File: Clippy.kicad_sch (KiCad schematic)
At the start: 17 parts, among them J1 Conn_01x08, SW1 PEC11R-4215F-S0024, U1 tiny2040, U2 SN74LV1T34DBV

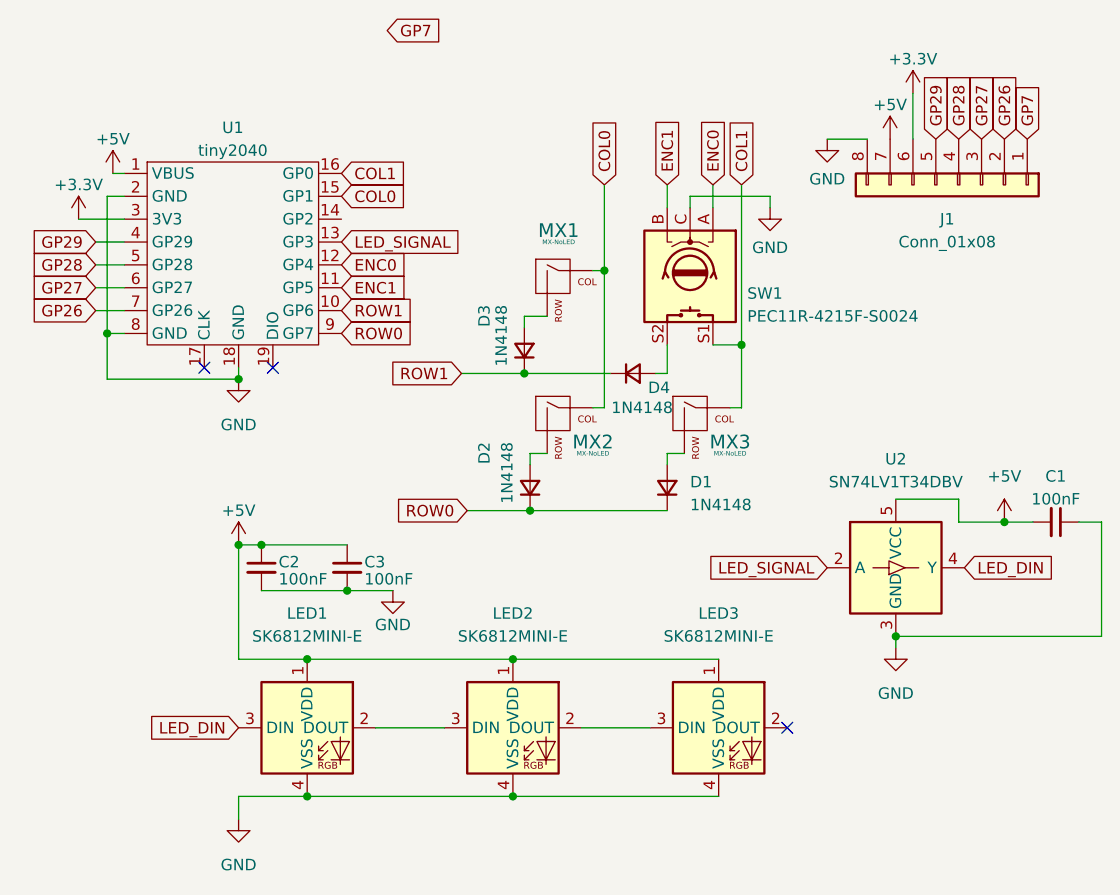
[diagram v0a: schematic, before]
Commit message: finishing touches 2 electric boogaloo
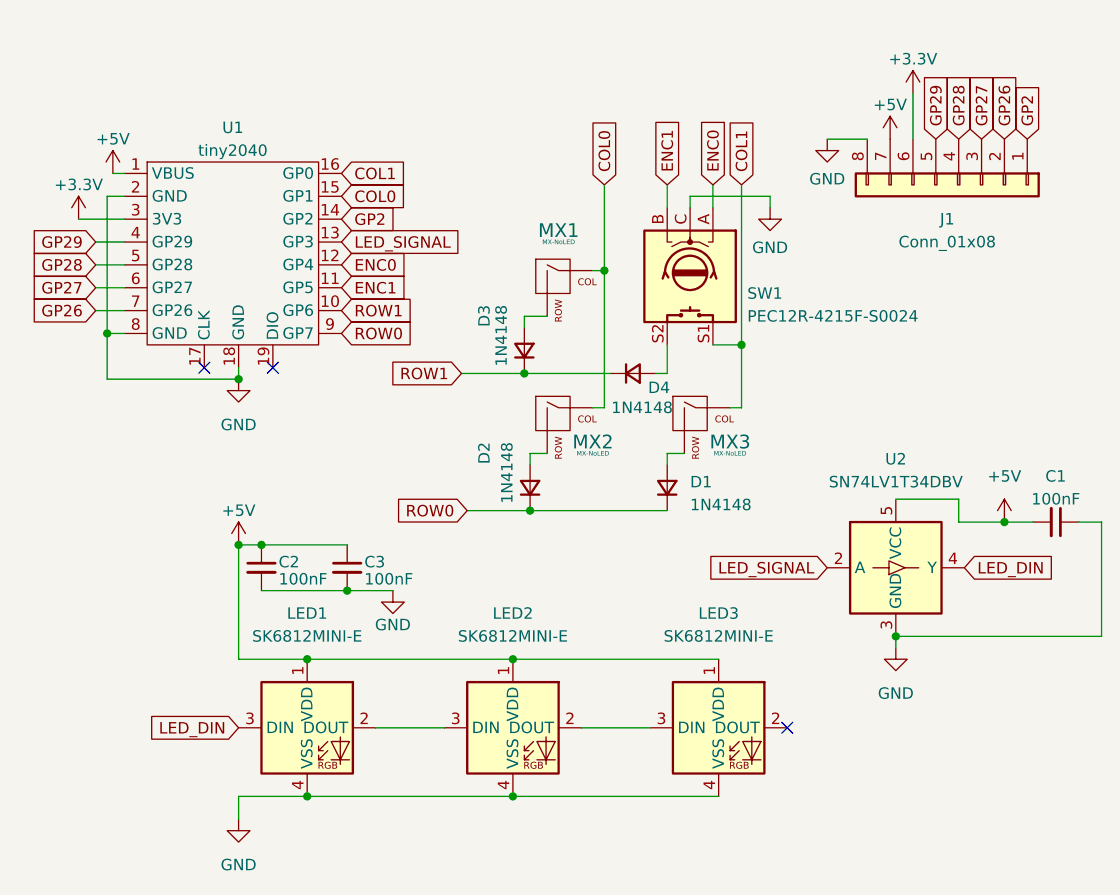
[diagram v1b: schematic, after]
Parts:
- C1, C2, C3: footprint Capacitor_SMD:C_0402_1005Metric_Pad0.74x0.62mm_HandSolder -> Capacitor_SMD:C_0805_2012Metric_Pad1.18x1.45mm_HandSolder
- SW1: value PEC11R-4215F-S0024 -> PEC12R-4215F-S0024
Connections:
- net GP7 is gone; now on net GP2: J1.1 (Pin_1)
- net GP2: now reaches U1.14 (GP2)
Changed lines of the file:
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@@
     (stroke (width 0) (type default))
   )
-  (global_label "GP7" (shape input) (at 191.135 78.74 90) (fields_autoplaced)
+  (global_label "GP2" (shape input) (at 191.135 78.74 90) (fields_autoplaced)
     (effects (font (size 1.27 1.27)) (justify left))
     (property "Intersheetrefs" "${INTERSHEET_REFS}" (at 191.135 72.0847 90)
@@
     )
   )
-  (global_label "GP7" (shape input) (at 120.015 66.675 0) (fields_autoplaced)
-    (effects (font (size 1.27 1.27)) (justify left))
-    (property "Intersheetrefs" "${INTERSHEET_REFS}" (at 126.6703 66.675 0)
+  (global_label "GP2" (shape input) (at 114.935 87.63 0) (fields_autoplaced)
+    (effects (font (size 1.27 1.27)) (justify left))
+    (property "Intersheetrefs" "${INTERSHEET_REFS}" (at 121.5903 87.63 0)
       (effects (font (size 1.27 1.27)) (justify left) hide)
     )
@@
       (effects (font (size 1.27 1.27)) (justify left))
     )
-    (property "Footprint" "Capacitor_SMD:C_0402_1005Metric_Pad0.74x0.62mm_HandSolder" (at 106.045 126.365 0)
+    (property "Footprint" "Capacitor_SMD:C_0805_2012Metric_Pad1.18x1.45mm_HandSolder" (at 106.045 126.365 0)
       (effects (font (size 1.27 1.27)) hide)
     )
@@
       (effects (font (size 1.27 1.27)) (justify left))
     )
-    (property "Value" "PEC11R-4215F-S0024" (at 160.02 98.425 90)
+    (property "Value" "PEC12R-4215F-S0024" (at 160.02 98.425 90)
       (effects (font (size 1.27 1.27)) (justify left))
     )
@@
       (effects (font (size 1.27 1.27)))
     )
-    (property "Footprint" "Capacitor_SMD:C_0402_1005Metric_Pad0.74x0.62mm_HandSolder" (at 194.31 121.285 0)
+    (property "Footprint" "Capacitor_SMD:C_0805_2012Metric_Pad1.18x1.45mm_HandSolder" (at 194.31 121.285 0)
       (effects (font (size 1.27 1.27)) hide)
     )
@@
       (effects (font (size 1.27 1.27)) (justify left))
     )
-    (property "Footprint" "Capacitor_SMD:C_0402_1005Metric_Pad0.74x0.62mm_HandSolder" (at 115.57 126.365 0)
-      (effects (font (size 1.27 1.27)) hide)
-    )
+    (property "Footprint" "Capacitor_SMD:C_0805_2012Metric_Pad1.18x1.45mm_HandSolder" (at 115.57 126.365 0)
+      (effects (font (size 1.27 1.27)) hide)
+    )
